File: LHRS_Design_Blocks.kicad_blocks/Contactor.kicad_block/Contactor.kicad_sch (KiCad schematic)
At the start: 25 parts

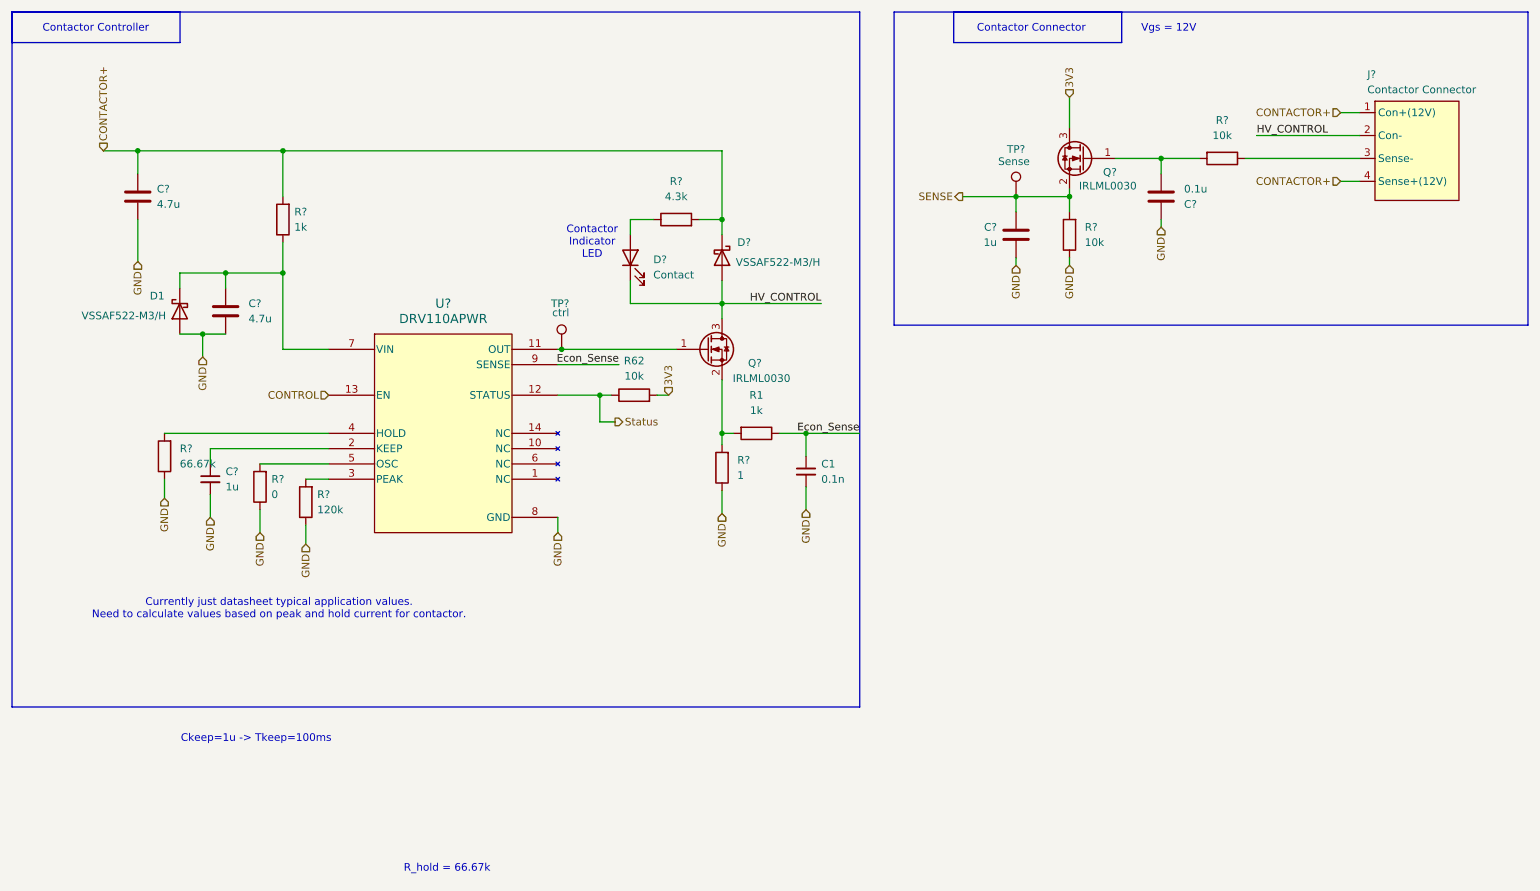
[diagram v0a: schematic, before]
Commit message: Rev a fixes (#84)
* updated buck block

* tp symbol + usb fixes

* fixes

* updated .gitignore

* updated conns
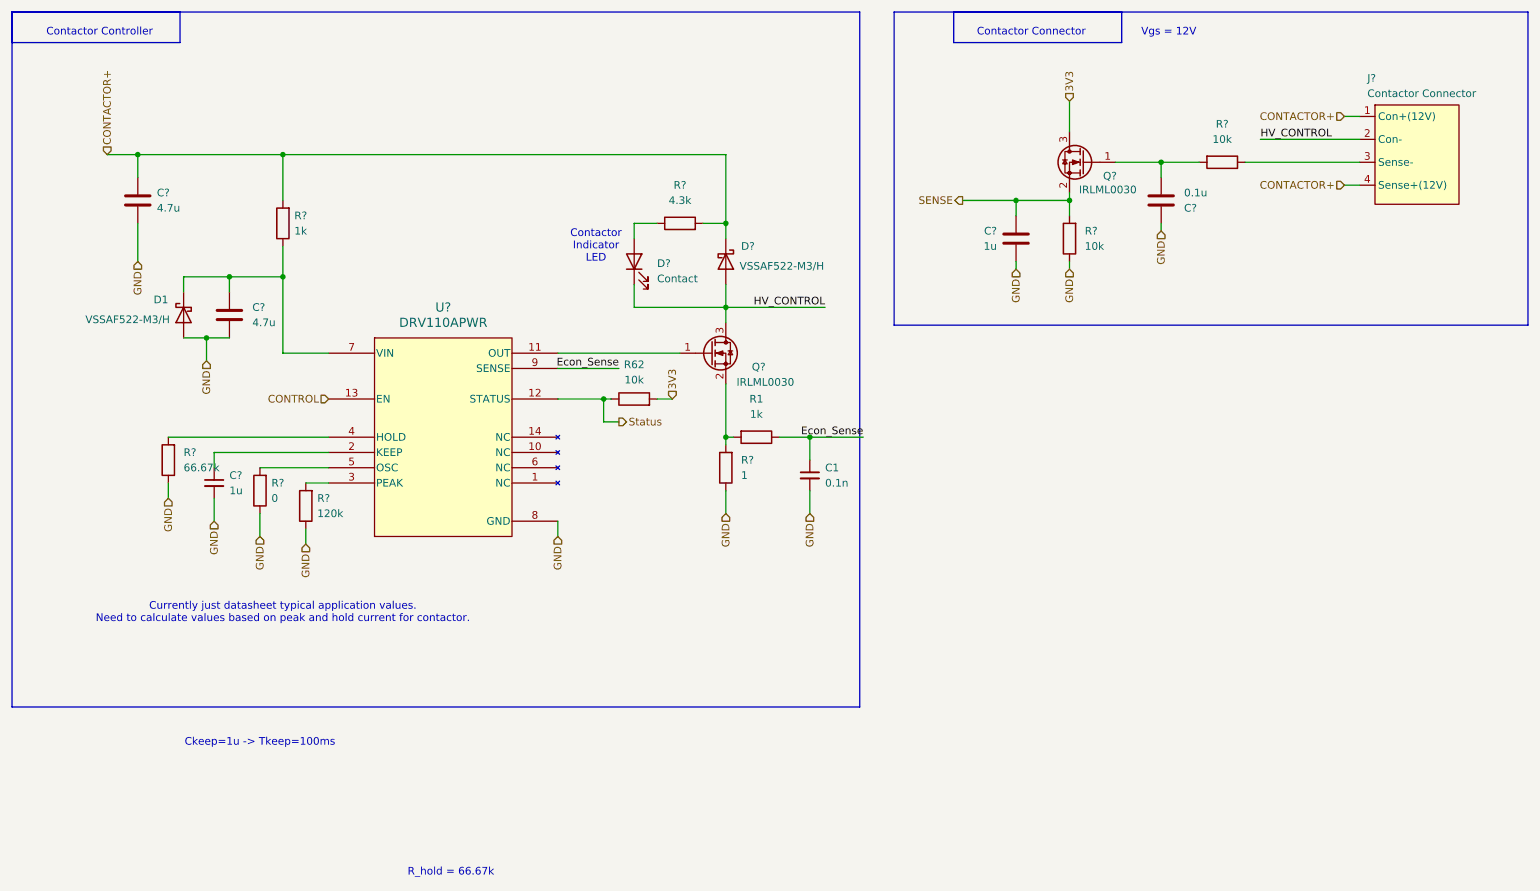
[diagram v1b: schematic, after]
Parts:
- removed TP?: ctrl, TestPoint:TestPoint_THTPad_D3.0mm_Drill1.5mm, symbol Connector:TestPoint
- removed TP?: Sense, TestPoint:TestPoint_THTPad_D3.0mm_Drill1.5mm, symbol Connector:TestPoint
- C?: LCSC P/N (none) -> C14663; Mouser Part Number 963-HMK107B7104KA-T -> (none)
- C?: Mouser Part Number 963-UMK107BJ105KA-T -> (none)
- D1, D?: LCSC P/N (none) -> C6326606; Manufactuerer Vishay General Semiconductor -> (none)
- D?: LCSC P/N (none) -> C84263; Manufactuerer NATIONSTAR -> (none)
- Q? (x2): LCSC P/N (none) -> C67272
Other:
- moved on the sheet: C1, C?, D1, D?, J?, Q?, R1, R62, R?, U?
